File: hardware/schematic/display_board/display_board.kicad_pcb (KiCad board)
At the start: 2 copper layers, 62 x 58.5 mm, 7 parts, among them J1 LINK, SW1 SW_Push, SW2 SW_Push

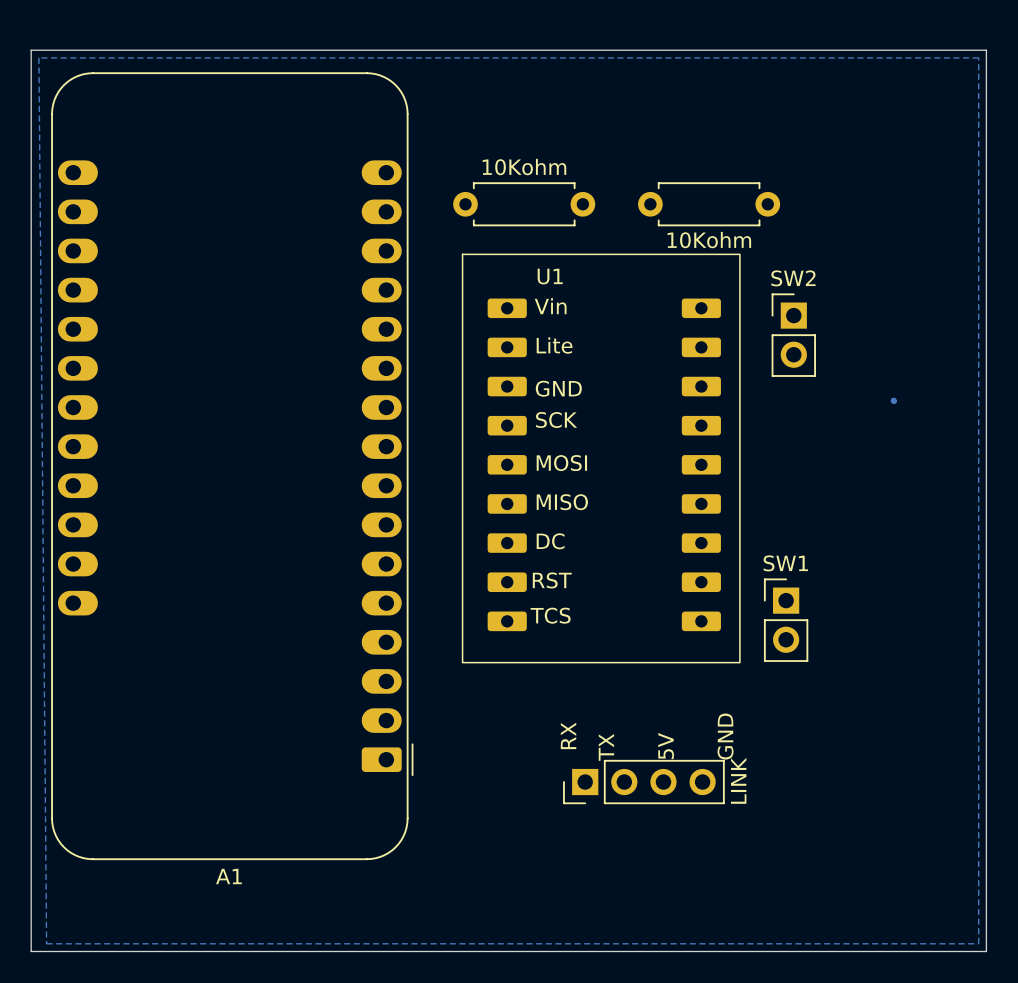
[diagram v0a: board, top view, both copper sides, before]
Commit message: First version of Nav PCB
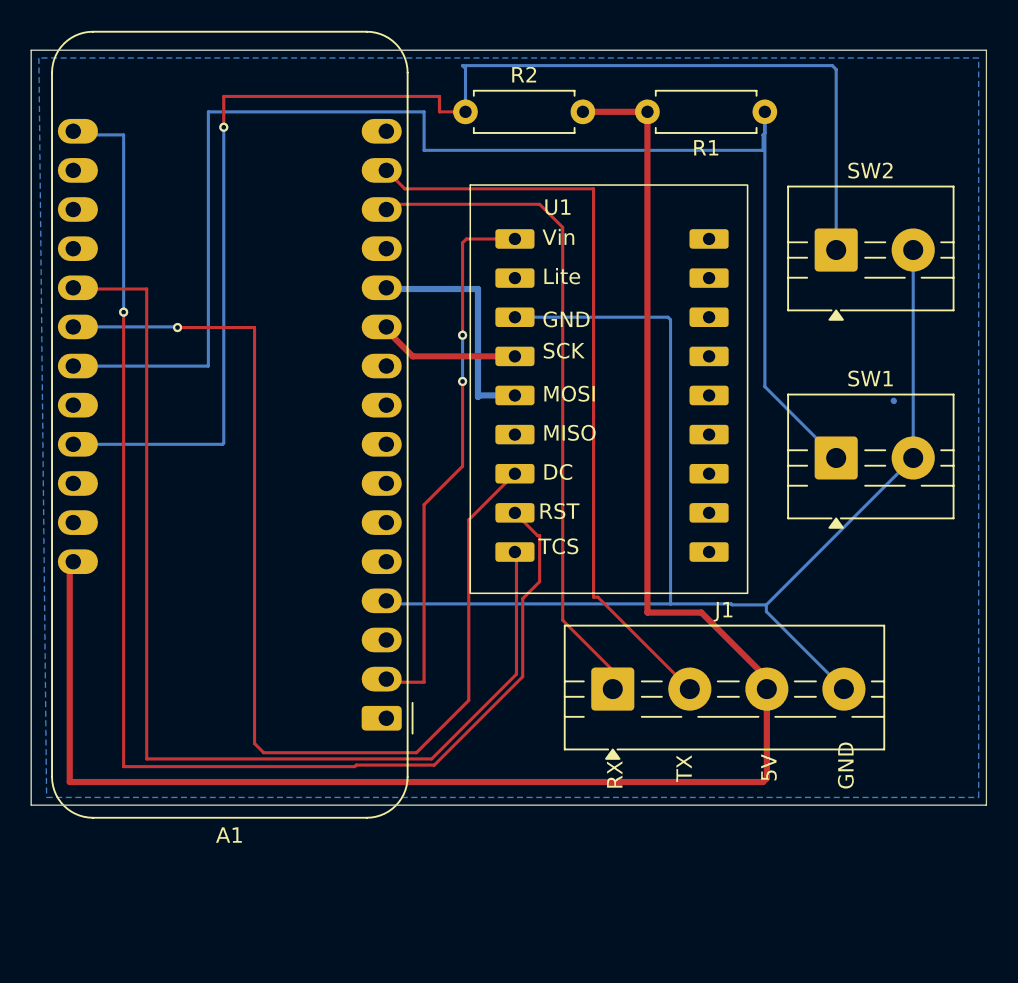
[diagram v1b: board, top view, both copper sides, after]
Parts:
- J1: value LINK -> Conn_01x04_Pin; footprint Connector_PinHeader_2.54mm:PinHeader_1x04_P2.54mm_Vertical -> TerminalBlock:TerminalBlock_MaiXu_MX126-5.0-04P_1x04_P5.00mm
- SW1, SW2: footprint Connector_PinHeader_2.54mm:PinHeader_1x02_P2.54mm_Vertical -> TerminalBlock:TerminalBlock_MaiXu_MX126-5.0-02P_1x02_P5.00mm
- moved SW1 9.81 mm to (138.2, 93.5)
- moved J1 6.29 mm to (123.8, 108.5), turned to 0 degrees
- moved R1 6.00 mm to (133.6, 71.0)
- moved R2 6.00 mm to (114.2, 71.0)
- moved SW2 5.07 mm to (138.2, 80.0)
- moved U1 4.53 mm to (117.4, 79.2)
- moved A1 2.69 mm to (109.1, 110.4)
- renumbered 10Kohm to R1, 10Kohm to R2
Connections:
- net Net-(A1-A8/IO15) renamed /DC
- net Net-(A1-SCK/IO5) renamed /MOSI
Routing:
- net +5V: track 0.00 -> 112.3 mm
- net Net-(A1-A10/IO27): track 0.00 -> 90.7 mm
- net Net-(A1-A12/IO13): track 0.00 -> 88.1 mm, vias 0 -> 1
- net GND: track 0.03 -> 87.9 mm
- net Net-(A1-SDA/IO23): track 0.00 -> 84.5 mm, vias 0 -> 1
- net Net-(A1-A9/IO33): track 0.00 -> 70.3 mm, vias 0 -> 1
- net /DC: track 0.00 -> 69.7 mm
- net Net-(A1-TX/IO17): track 0.00 -> 49.2 mm
- net Net-(A1-RX/IO16): track 0.00 -> 44.2 mm
- net /3V3: track 0.00 -> 35.8 mm, vias 0 -> 2
- net Net-(A1-MOSI/IO18): track 0.00 -> 15.4 mm
- net /MOSI: track 0.00 -> 9.05 mm
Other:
- board size 62 x 58.5 mm -> 62 x 49 mm
